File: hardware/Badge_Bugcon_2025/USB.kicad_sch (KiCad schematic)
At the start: 37 parts, among them J10 Battery, J3 USB_A, J4 USB_A, J6 USB_A, P4 USB_C_Plug_USB2.0, Q1 DMG3415U-7, SW1 ON, SW4 On, U1 USB3740B-AI9, U3 SL2.1A, U5 MCP73831T-2ATI/OT, Y5 12MHz

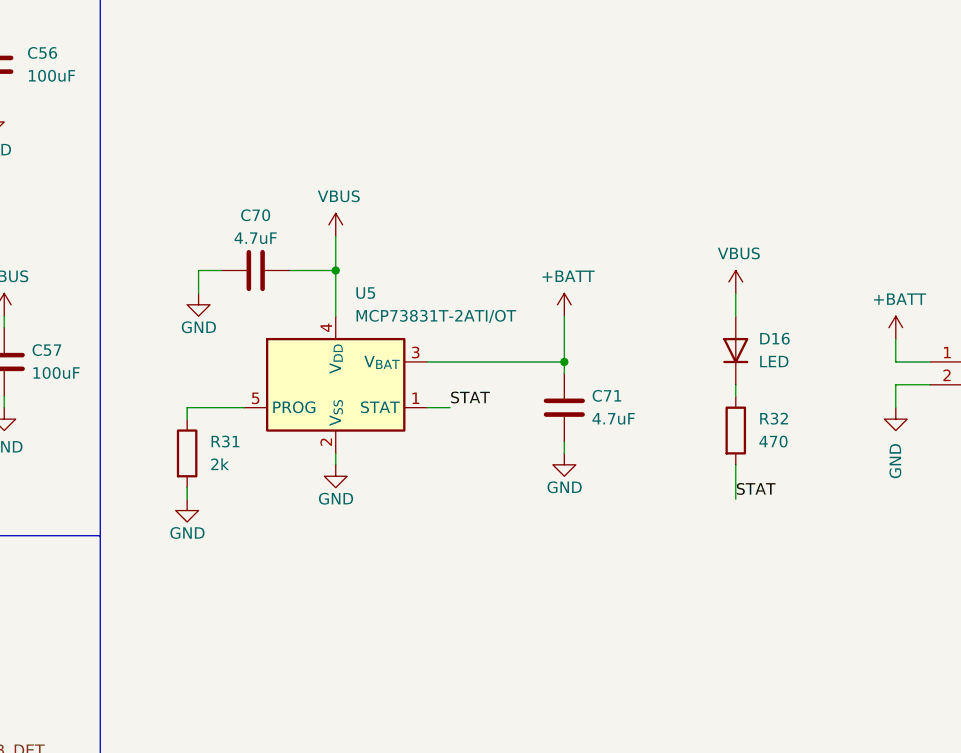
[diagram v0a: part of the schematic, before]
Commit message: feat(Hw):Update_Schematic
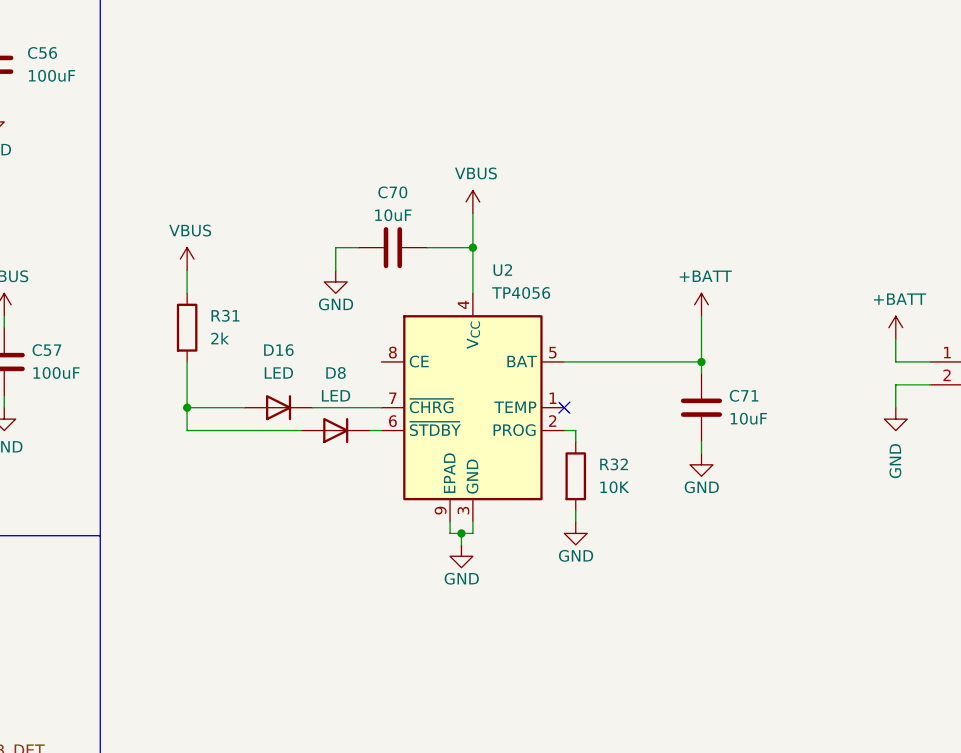
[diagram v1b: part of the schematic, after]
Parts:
- removed U5: MCP73831T-2ATI/OT, Package_TO_SOT_SMD:SOT-23-5, symbol Battery_Management:MCP73831-2-OT
- added D8: LED, LED_SMD:LED_0603_1608Metric, symbol Device:D
- added U2: TP4056, Package_SO:SOIC-8-1EP_3.9x4.9mm_P1.27mm_EP2.41x3.3mm_ThermalVias, symbol Battery_Management:TP4056-42-ESOP8
- C70, C71: value 4.7uF -> 10uF
- R32: value 470 -> 10K; footprint LED_SMD:LED_0603_1608Metric -> Resistor_SMD:R_0402_1005Metric; LCSC# C23179 -> C2759535
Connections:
- net STAT is gone; now on net GND: R32.2
- net +BATT: now also U2.5 (BAT)
- net GND: now also U2.3 (GND), U2.9 (EPAD); no longer R31.2
- net VBUS: now also R31.1, U2.4 (V_{CC}); no longer D16.2 (A)
- net at D16.1 (K): now also U2.7 (~{CHRG}); no longer R32.1
- new net: D16.2 (A), D8.2 (A), R31.2
- new net: R32.1, U2.2 (PROG)
- new net: D8.1 (K), U2.6 (~{STDBY})
- no-connect marks 4 -> 5
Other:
- moved on the sheet: C70, C71, D16, R31
